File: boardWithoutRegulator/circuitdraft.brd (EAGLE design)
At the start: 64.4 x 41 mm, 36 parts, among them IC1 BQ25887RGER, Q1 16 MHz

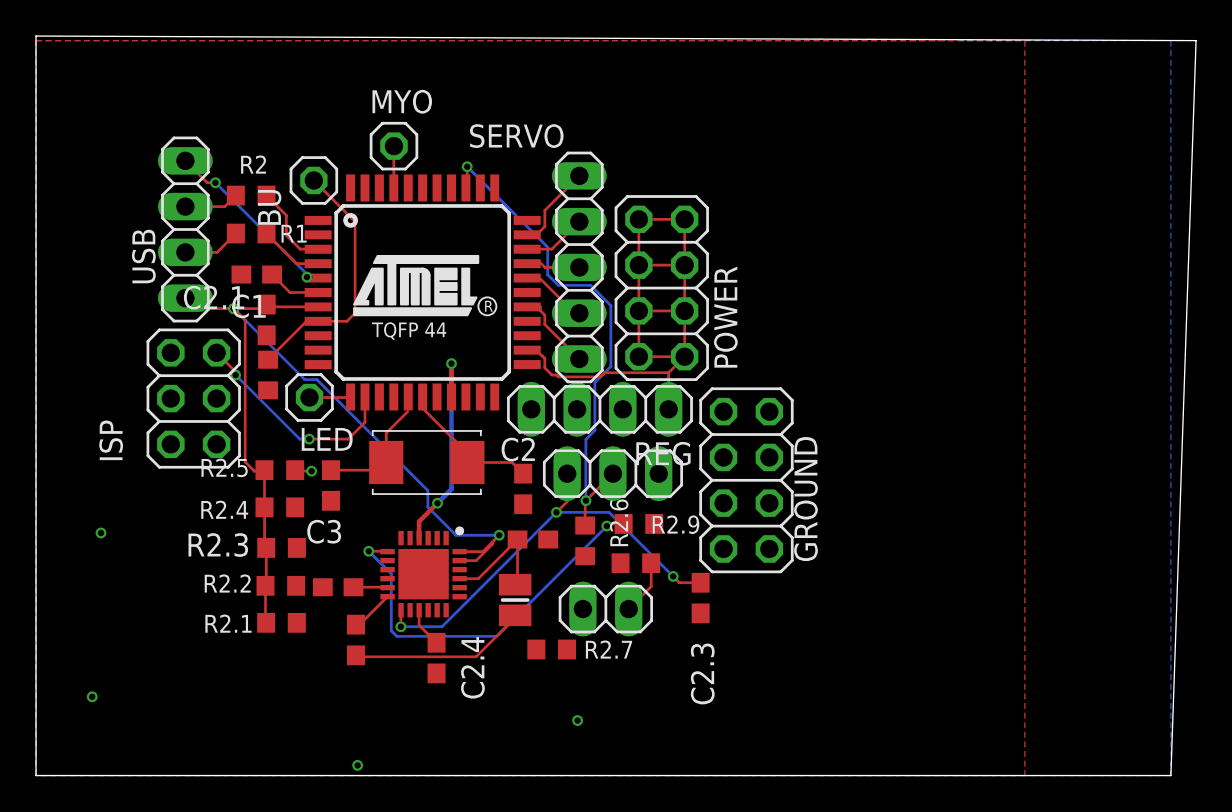
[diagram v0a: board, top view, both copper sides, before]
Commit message: Ahmad's suggestions
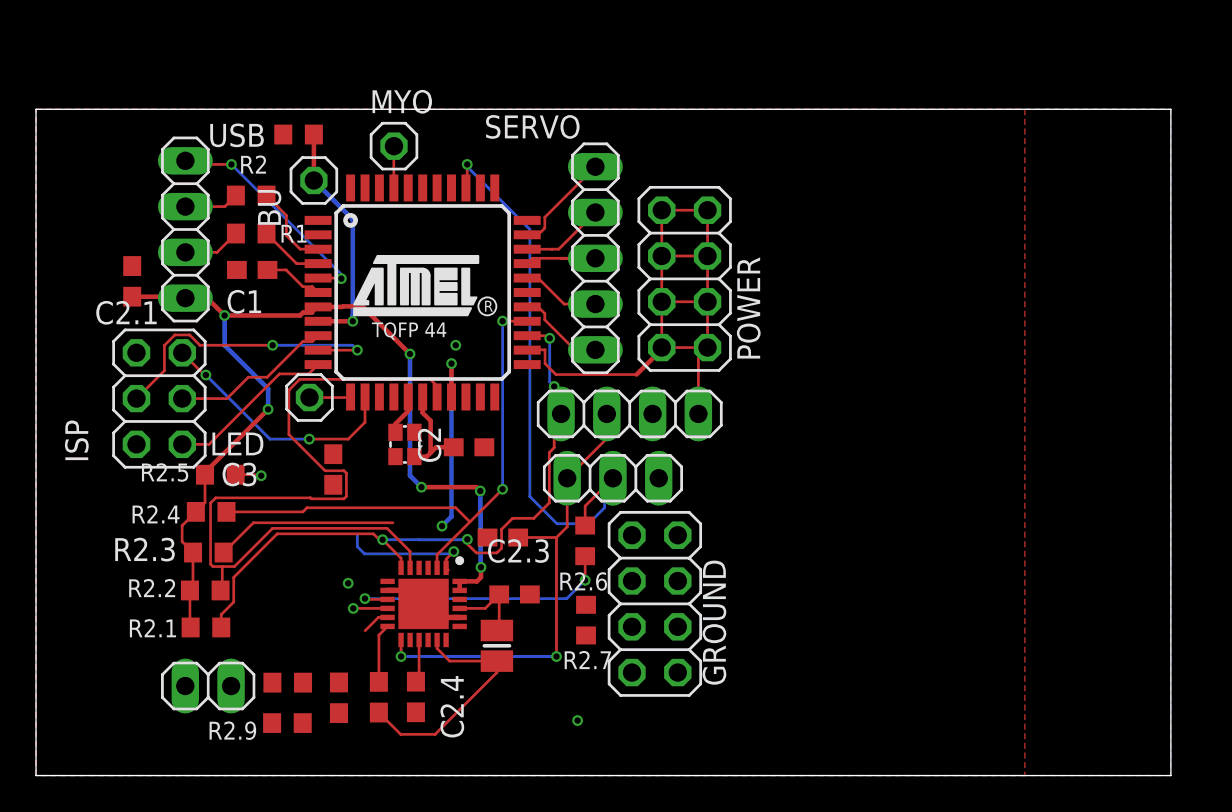
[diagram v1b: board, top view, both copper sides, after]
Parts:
- Q1: device SamacSys_Parts:ECS2501823GJGNTR -> crystal-geyer_V1_0:2.0X1.6_KX-5
- moved TS 22.5 mm to (20.6, 4.97)
- moved R2.9 22.4 mm to (24.9, 2.91)
- moved R2.8 20.4 mm to (25.0, 5.16), turned to 0 degrees
- moved RBUTTON 13.5 mm to (25.6, 35.6), turned to 180 degrees
- moved C2.3 11.5 mm to (36.9, 13.2), turned to 0 degrees
- moved GROUND 8.53 mm to (45.3, 9.53)
- moved C2.1 7.76 mm to (16.3, 27.4), turned to 270 degrees
- moved C2.2 6.14 mm to (27.8, 4.32), turned to 270 degrees
- moved R2.1 4.20 mm to (20.4, 8.22)
- moved R2.2 4.20 mm to (20.4, 10.3)
- moved R2.3 4.07 mm to (20.6, 12.4)
- moved R2.4 3.82 mm to (20.7, 14.6)
- moved C2 3.79 mm to (35.0, 18.2), turned to 180 degrees
- moved C2.5 3.42 mm to (30.0, 4.35)
- moved R2.5 3.31 mm to (21.2, 16.7)
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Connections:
- net N$6: now also Q1.3; no longer Q1.2
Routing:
- net SCL: track 0.00 -> 43.0 mm
- net INT: track 0.00 -> 36.9 mm, vias 0 -> 4
- net STAT: track 0.00 -> 30.5 mm, vias 0 -> 2
- net TS: track 24.6 -> 1.02 mm, vias 2 -> 0
- net MOSI: track 0.00 -> 17.1 mm, vias 0 -> 2
- net N$10: track 0.00 -> 15.3 mm, vias 0 -> 2
- net MISO: track 0.00 -> 9.37 mm
- net SCK: track 0.00 -> 8.98 mm
- net SDA: track 12.3 -> 21.2 mm
- net N$7: track 0.93 -> 9.10 mm, vias 1 -> 2
- net GND: track 0.00 -> 4.62 mm, vias 0 -> 2
- net N$5: track 6.56 -> 2.25 mm
- net SIGNAL2: track 2.26 -> 5.81 mm
- net MIDDLE: track 28.2 -> 31.5 mm, vias 2 -> 1
- net N$18: track 9.90 -> 13.2 mm
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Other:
- board size 64.4 x 41 mm -> 63 x 37 mm
